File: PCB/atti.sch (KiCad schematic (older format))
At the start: 38 parts, among them J1 Conn_02x04_Counter_Clockwise, J2 Conn_01x01_Female, J3 Conn_01x01_Female, J4 Conn_01x01_Female, J5 Conn_01x01_Female, J6 Conn_01x01_Female, J7 Conn_01x01_Female, J8 Conn_01x01_Female, J9 Conn_01x01_Female, SW1 SW_SPST, U1 AP2112K-3.3, U2 STM32F303K8Tx, U3 NVT2006, U5 BMX160, U6 BMP280, Y1 32 MHz

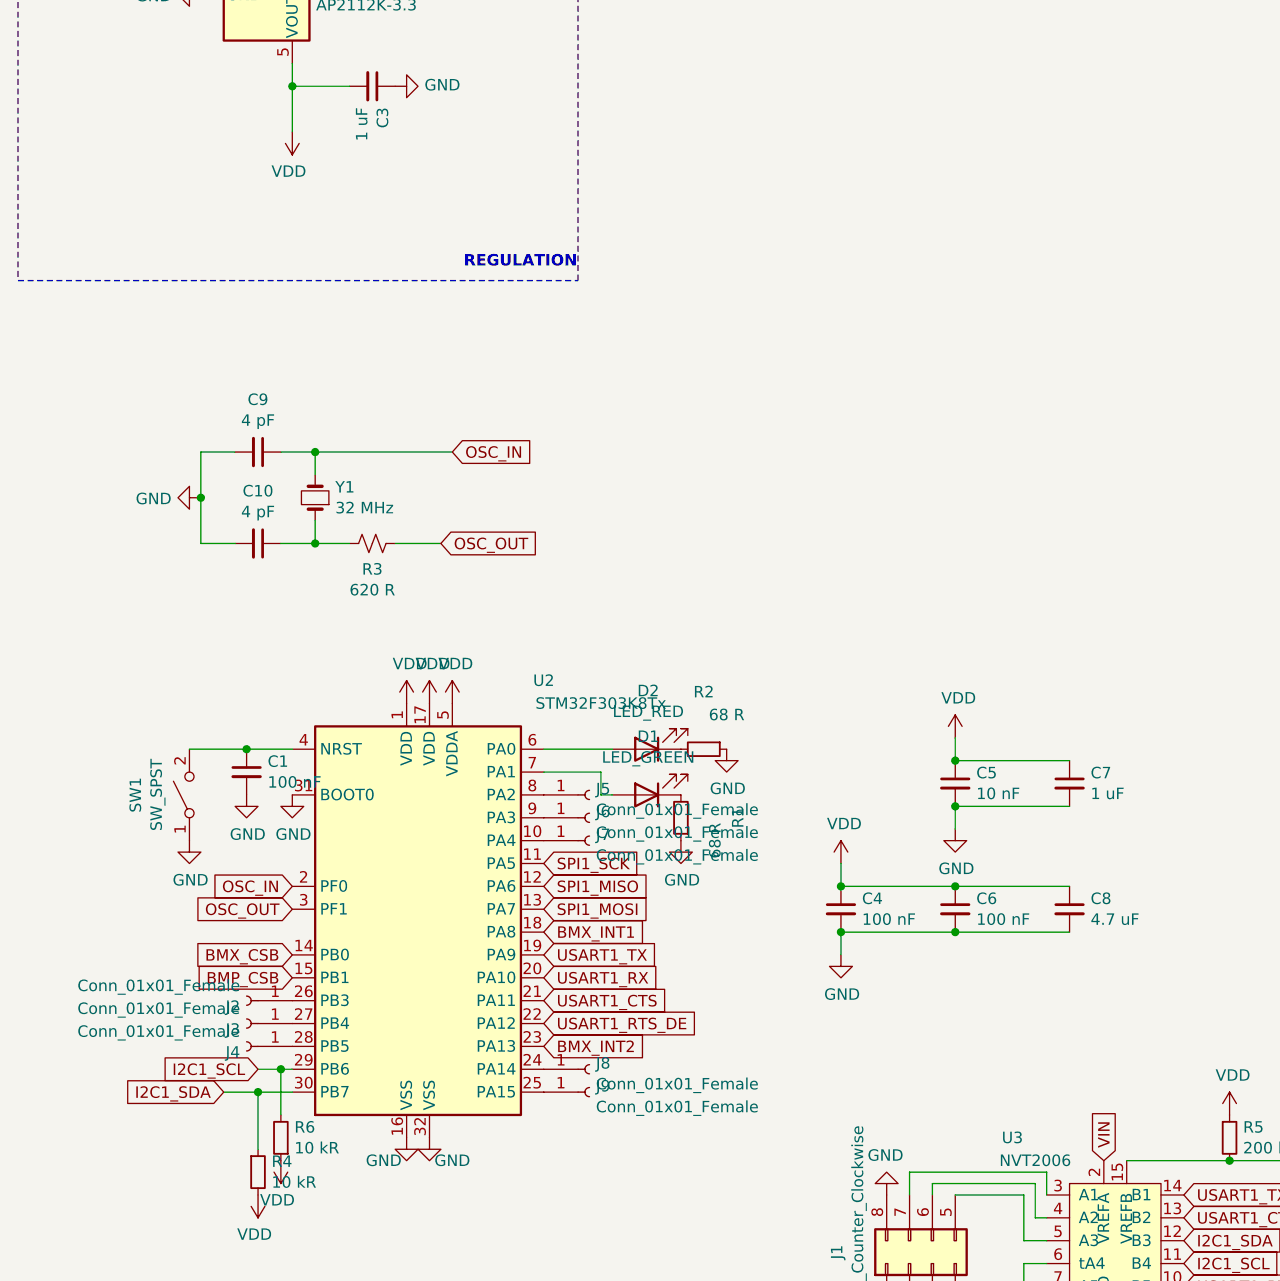
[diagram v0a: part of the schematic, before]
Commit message: Partial routing attempt and programming connector
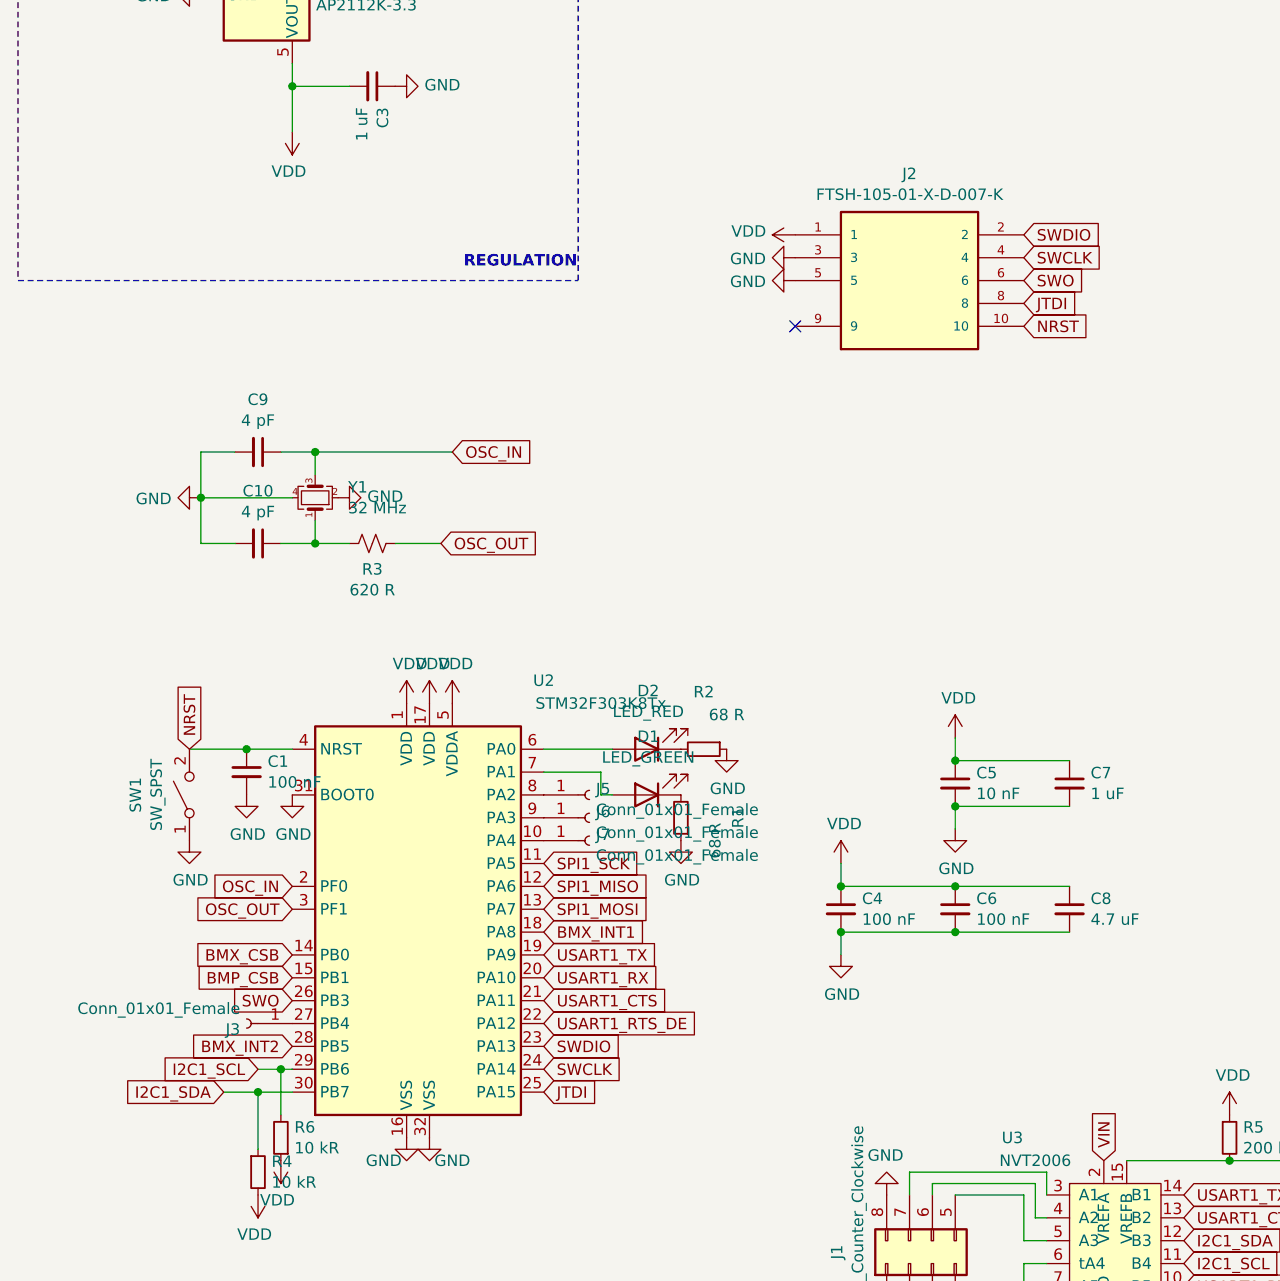
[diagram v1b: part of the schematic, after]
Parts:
- removed J2, J4, J8, J9: Conn_01x01_Female, Connector_Wire:SolderWire-0.25sqmm_1x01_D0.65mm_OD1.7mm, symbol Connector:Conn_01x01_Female
- removed Y1: 32 MHz, Crystal:Crystal_SMD_SeikoEpson_TSX3225-4Pin_3.2x2.5mm, symbol Device:Crystal_Small
- added J2: FTSH-105-01-X-D-007-K, AsymConnectors:SAMTEC_FTSH-105-01-X-D-007-K, symbol AsymConnectors:FTSH-105-01-X-D-007-K
- added Y1: 32 MHz, Crystal:Crystal_SMD_SeikoEpson_TSX3225-4Pin_3.2x2.5mm, symbol Device:Crystal_GND24_Small
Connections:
- net BMX_INT2: now also U2.28 (PB5); no longer U2.23 (PA13)
- net GND: now also J2.3, J2.5, Y1.2, Y1.4
- net OSC_IN: now also Y1.3
- net VDD: now also J2.1
- net SWCLK: now reaches U2.24 (PA14)
- net SWCLK: now also J2.4
- net JTDI: now reaches U2.25 (PA15)
- net JTDI: now also J2.8
- net SWO: now reaches U2.26 (PB3)
- net SWO: now also J2.6
- net NRST: now reaches C1.1, SW1.2 (B), U2.4 (NRST)
- net NRST: now also J2.10
- net at C10.1, R3.1: now also Y1.1
- new net SWDIO: J2.2, U2.23 (PA13)
- no-connect marks 0 -> 1
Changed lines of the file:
@@
 Text GLabel 2850 5500 2    50   Input ~ 0
 BMX_INT1
-Text GLabel 2850 6000 2    50   Input ~ 0
-BMX_INT2
 $Comp
 L AsymLevelShifters:NVT2006 U3
@@
 Wire Wire Line
 	3100 4800 3100 4900
-$Comp
-L Device:Crystal_Small Y1
-U 1 1 5FE3AFDC
-P 1850 3600
-F 0 "Y1" V 1896 3512 50  0000 R CNN
-F 1 "32 MHz" V 1805 3512 50  0000 R CNN
-F 2 "Crystal:Crystal_SMD_SeikoEpson_TSX3225-4Pin_3.2x2.5mm" H 1850 3600 50  0001 C CNN
-F 3 "~" H 1850 3600 50  0001 C CNN
-	1    1850 3600
-	0    -1   -1   0
-$EndComp
 Text GLabel 1750 5300 0    50   Input ~ 0
 OSC_IN
@@
 	2850 4800 3100 4800
 $Comp
-L Connector:Conn_01x01_Female J2
-U 1 1 5FE07EBD
-P 1550 5800
-F 0 "J2" H 1578 5826 50  0000 L CNN
-F 1 "Conn_01x01_Female" H 1578 5735 50  0000 L CNN
-F 2 "Connector_Wire:SolderWire-0.25sqmm_1x01_D0.65mm_OD1.7mm" H 1550 5800 50  0001 C CNN
-F 3 "~" H 1550 5800 50  0001 C CNN
-	1    1550 5800
-	-1   0    0    1
-$EndComp
-$Comp
 L Connector:Conn_01x01_Female J3
 U 1 1 5FE09C11
@@
 $EndComp
 $Comp
-L Connector:Conn_01x01_Female J4
-U 1 1 5FE0B773
-P 1550 6000
-F 0 "J4" H 1578 6026 50  0000 L CNN
-F 1 "Conn_01x01_Female" H 1578 5935 50  0000 L CNN
-F 2 "Connector_Wire:SolderWire-0.25sqmm_1x01_D0.65mm_OD1.7mm" H 1550 6000 50  0001 C CNN
-F 3 "~" H 1550 6000 50  0001 C CNN
-	1    1550 6000
-	-1   0    0    1
-$EndComp
-$Comp
-L Connector:Conn_01x01_Female J8
-U 1 1 5FE36D10
-P 3050 6100
-F 0 "J8" H 3078 6126 50  0000 L CNN
-F 1 "Conn_01x01_Female" H 3078 6035 50  0000 L CNN
-F 2 "Connector_Wire:SolderWire-0.25sqmm_1x01_D0.65mm_OD1.7mm" H 3050 6100 50  0001 C CNN
-F 3 "~" H 3050 6100 50  0001 C CNN
-	1    3050 6100
-	1    0    0    -1
-$EndComp
-$Comp
-L Connector:Conn_01x01_Female J9
-U 1 1 5FE38A2A
-P 3050 6200
-F 0 "J9" H 3078 6226 50  0000 L CNN
-F 1 "Conn_01x01_Female" H 3078 6135 50  0000 L CNN
-F 2 "Connector_Wire:SolderWire-0.25sqmm_1x01_D0.65mm_OD1.7mm" H 3050 6200 50  0001 C CNN
-F 3 "~" H 3050 6200 50  0001 C CNN
-	1    3050 6200
-	1    0    0    -1
-$EndComp
+L Device:Crystal_GND24_Small Y1
+U 1 1 5FE91EF3
+P 1850 3600
+F 0 "Y1" V 1896 3456 50  0000 R CNN
+F 1 "32 MHz" V 1805 3456 50  0000 R CNN
+F 2 "Crystal:Crystal_SMD_SeikoEpson_TSX3225-4Pin_3.2x2.5mm" H 1850 3600 50  0001 C CNN
+F 3 "~" H 1850 3600 50  0001 C CNN
+	1    1850 3600
+	0    -1   -1   0
+$EndComp
+Wire Wire Line
+	1750 3600 1350 3600
+$Comp
+L power:GND #PWR?
+U 1 1 5FE9FB52
+P 1950 3600
+F 0 "#PWR?" H 1950 3350 50  0001 C CNN
+F 1 "GND" V 1955 3472 50  0000 R CNN
+F 2 "" H 1950 3600 50  0001 C CNN
+F 3 "" H 1950 3600 50  0001 C CNN
+	1    1950 3600
+	0    -1   -1   0
+$EndComp
+Text GLabel 1750 5800 0    50   Input ~ 0
+SWO
+Text GLabel 1750 6000 0    50   Input ~ 0
+BMX_INT2
+Text GLabel 2850 6000 2    50   Input ~ 0
+SWDIO
+Text GLabel 2850 6100 2    50   Input ~ 0
+SWCLK
+Text GLabel 1300 4700 1    50   Input ~ 0
+NRST
+Text GLabel 2850 6200 2    50   Input ~ 0
+JTDI
+Text GLabel 4950 2450 2    50   Input ~ 0
+SWDIO
+Text GLabel 4950 2550 2    50   Input ~ 0
+SWCLK
+Text GLabel 4950 2650 2    50   Input ~ 0
+SWO
+Text GLabel 4950 2750 2    50   Input ~ 0
+JTDI
+Text GLabel 4950 2850 2    50   Input ~ 0
+NRST
+$Comp
+L power:VDD #PWR?
+U 1 1 60088F29
+P 3950 2450
+F 0 "#PWR?" H 3950 2300 50  0001 C CNN
+F 1 "VDD" V 3965 2577 50  0000 L CNN
+F 2 "" H 3950 2450 50  0001 C CNN
+F 3 "" H 3950 2450 50  0001 C CNN
+	1    3950 2450
+	0    -1   -1   0
+$EndComp
+$Comp
+L power:GND #PWR?
+U 1 1 60089B95
+P 3950 2550
+F 0 "#PWR?" H 3950 2300 50  0001 C CNN
+F 1 "GND" V 3955 2422 50  0000 R CNN
+F 2 "" H 3950 2550 50  0001 C CNN
+F 3 "" H 3950 2550 50  0001 C CNN
+	1    3950 2550
+	0    1    1    0
+$EndComp
+$Comp
+L power:GND #PWR?
+U 1 1 6008A5E8
+P 3950 2650
+F 0 "#PWR?" H 3950 2400 50  0001 C CNN
+F 1 "GND" V 3955 2522 50  0000 R CNN
+F 2 "" H 3950 2650 50  0001 C CNN
+F 3 "" H 3950 2650 50  0001 C CNN
+	1    3950 2650
+	0    1    1    0
+$EndComp
+NoConn ~ 3950 2850
+$Comp
+L AsymConnectors:FTSH-105-01-X-D-007-K J2
+U 1 1 6009A82F
+P 4450 2650
+F 0 "J2" H 4450 3117 50  0000 C CNN
+F 1 "FTSH-105-01-X-D-007-K" H 4450 3026 50  0000 C CNN
+F 2 "AsymConnectors:SAMTEC_FTSH-105-01-X-D-007-K" H 4250 3200 50  0001 L BNN
+F 3 "" H 4700 2950 50  0001 L BNN
+F 4 "SAMTEC" H 4250 3100 50  0001 L BNN "MANUFACTURER"
+F 5 "B" H 4700 3000 50  0001 L BNN "PARTREV"
+F 6 "Manufacturer Recommendations" H 4250 3300 50  0001 L BNN "STANDARD"
+F 7 "5.7mm" H 4250 3000 50  0001 L BNN "MAXIMUM_PACKAGE_HEIGHT"
+	1    4450 2650
+	1    0    0    -1
+$EndComp

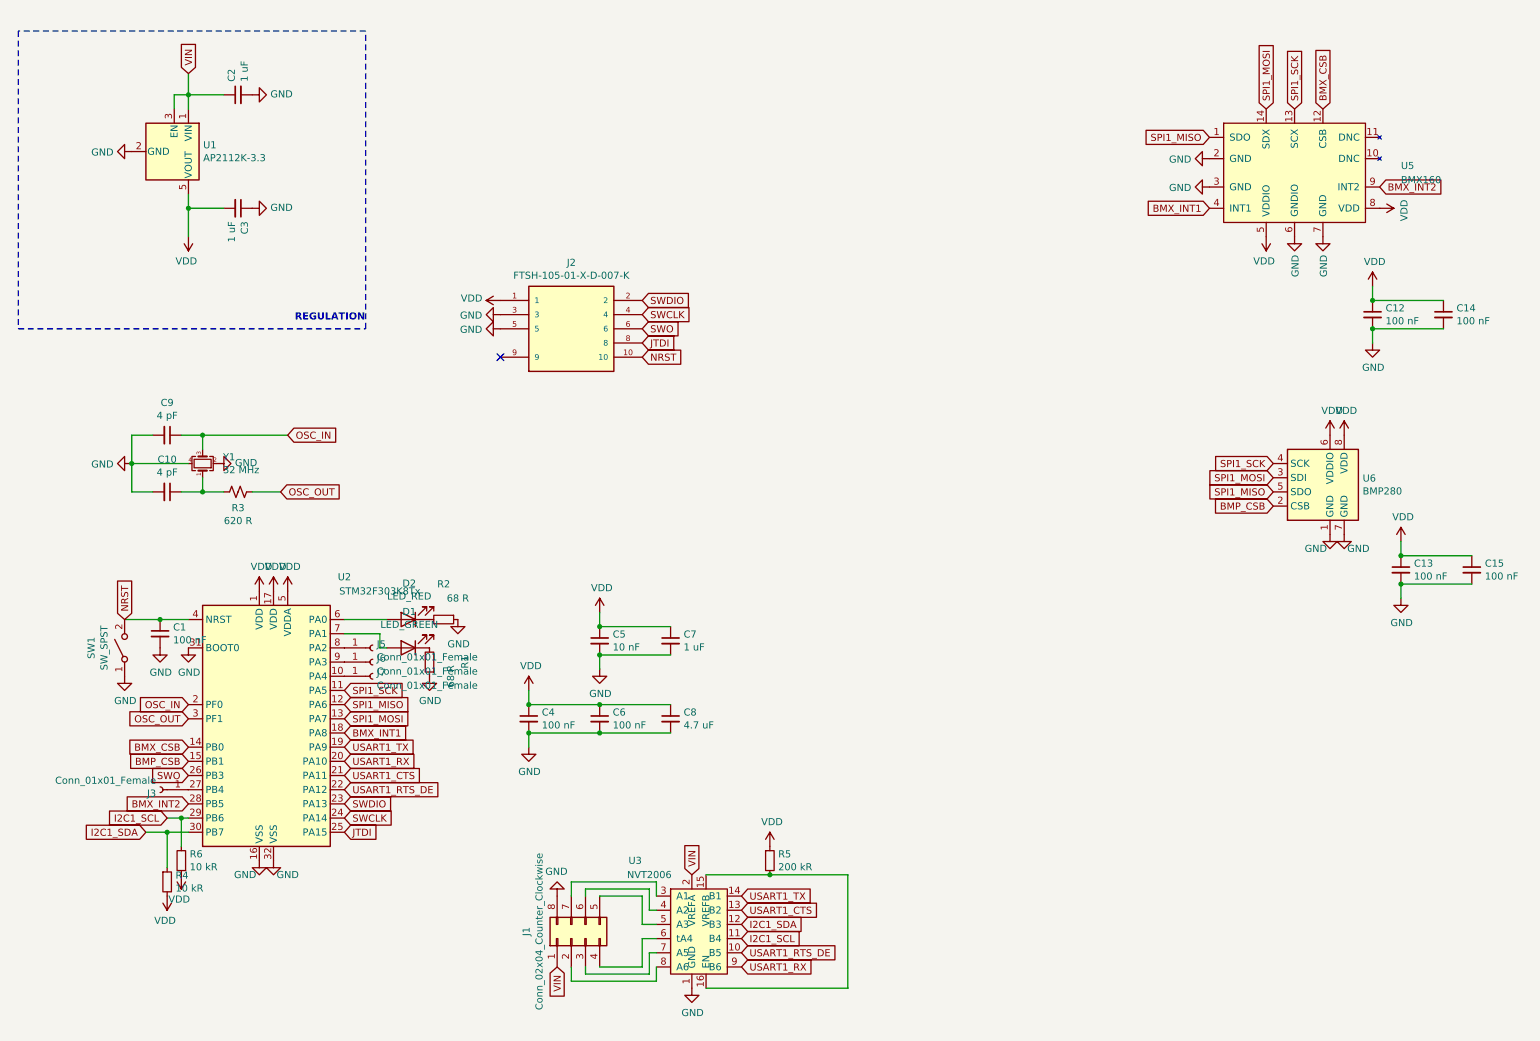
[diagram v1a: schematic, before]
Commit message: Second routing attempt
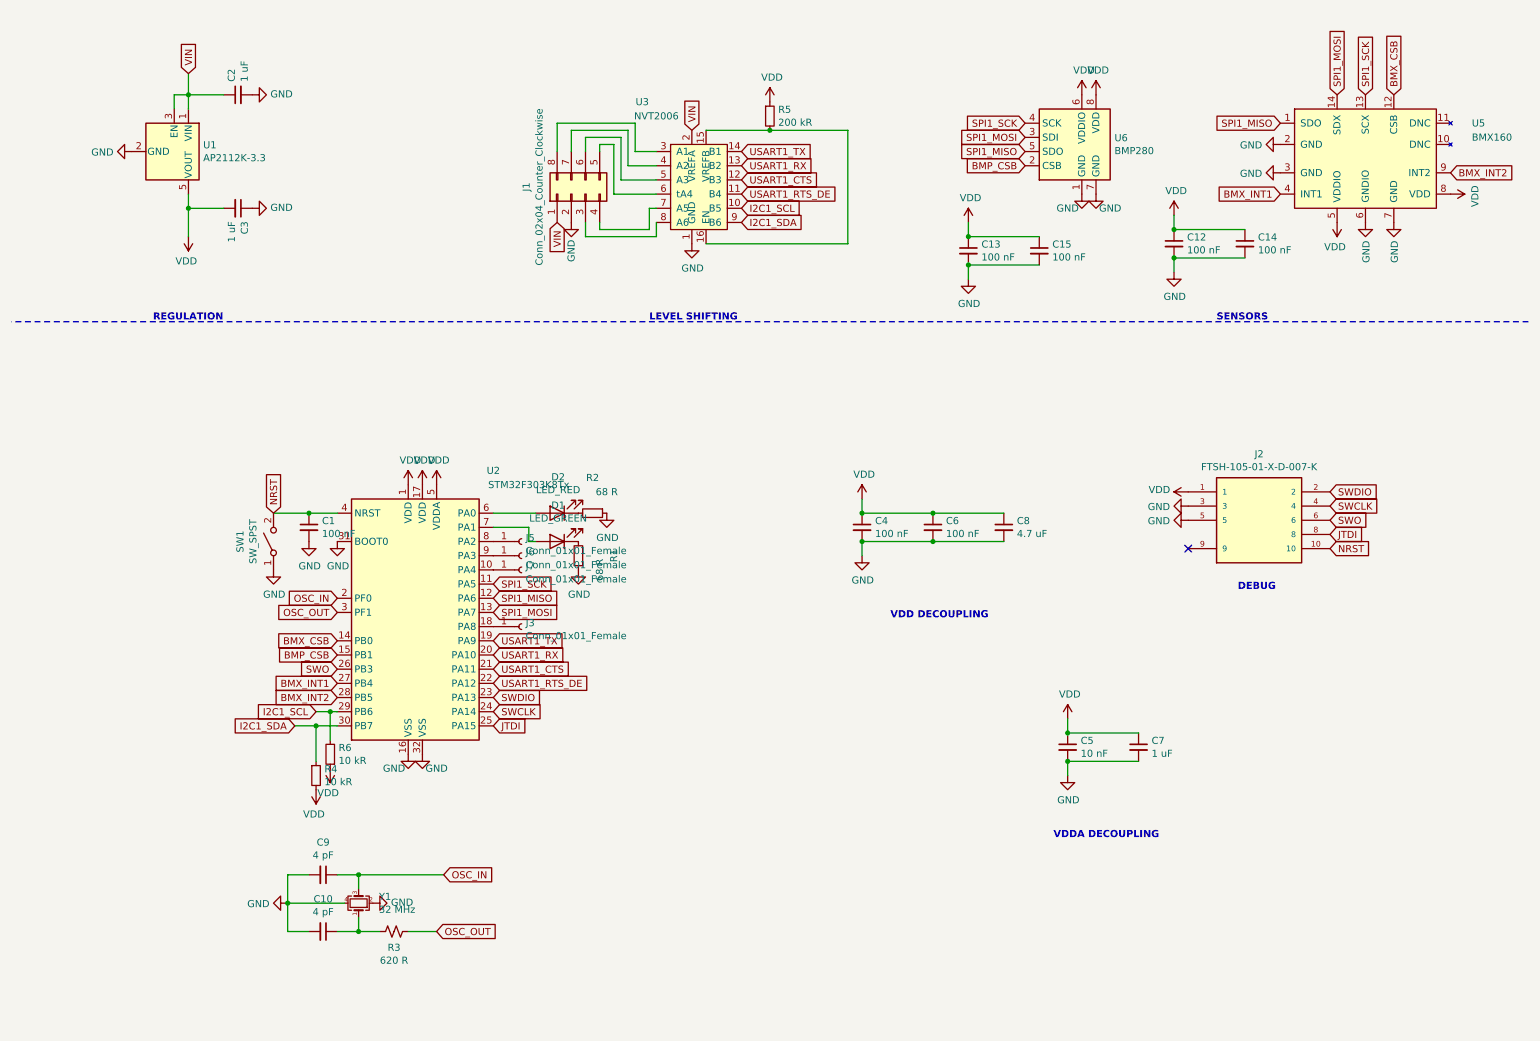
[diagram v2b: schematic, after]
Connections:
- net BMX_INT1: now also U2.27 (PB4); no longer U2.18 (PA8)
- net GND: now also J1.2 (Pin_2); no longer J1.8 (Pin_8)
- net I2C1_SCL: now also U3.10 (B5); no longer U3.11 (B4)
- net I2C1_SDA: now also U3.9 (B6); no longer U3.12 (B3)
- net USART1_CTS: now also U3.12 (B3); no longer U3.13 (B2)
- net USART1_RTS_DE: now also U3.11 (B4); no longer U3.10 (B5)
- net USART1_RX: now also U3.13 (B2); no longer U3.9 (B6)
- net at J3.1 (Pin_1): now also U2.18 (PA8); no longer U2.27 (PB4)
- net at U3.8 (A6): now also J1.3 (Pin_3); no longer J1.2 (Pin_2)
- net at U3.7 (A5): now also J1.4 (Pin_4); no longer J1.3 (Pin_3)
- net at U3.6 (tA4): now also J1.5 (Pin_5); no longer J1.4 (Pin_4)
- net at U3.5 (A3): now also J1.6 (Pin_6); no longer J1.5 (Pin_5)
- net at U3.4 (A2): now also J1.7 (Pin_7); no longer J1.6 (Pin_6)
- net at U3.3 (A1): now also J1.8 (Pin_8); no longer J1.7 (Pin_7)
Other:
- note added: "DEBUG"
- note added: "LEVEL SHIFTING"
- note added: "SENSORS"
- note added: "VDD DECOUPLING"
- note added: "VDDA DECOUPLING"
- moved on the sheet: C1, C10, C12, C13, C14, C15, C4, C5, C6, C7, C8, C9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
